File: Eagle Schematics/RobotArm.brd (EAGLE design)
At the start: 54.5 x 52.6 mm, 86 parts, among them J1 5A/28V, SW1 5A/28V

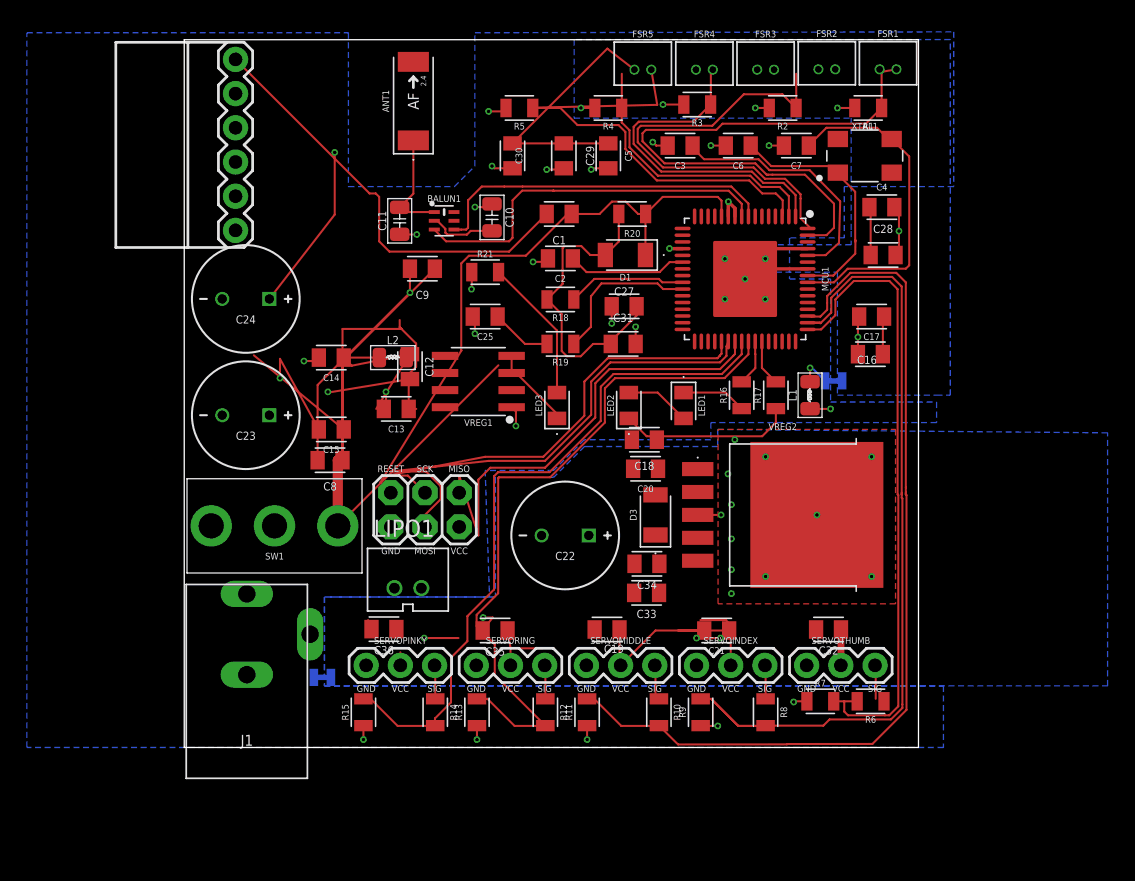
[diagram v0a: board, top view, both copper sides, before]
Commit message: reorganized
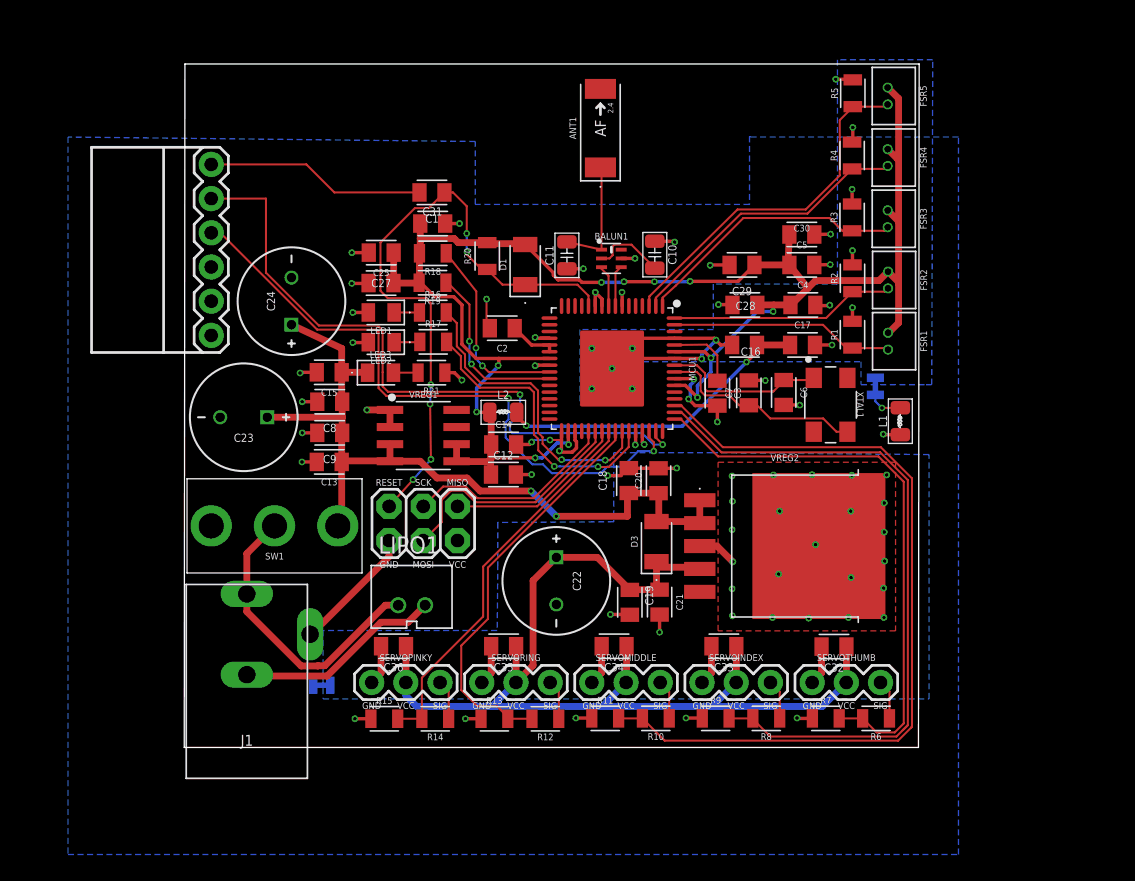
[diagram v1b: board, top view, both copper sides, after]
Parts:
- moved R17 25.8 mm to (18.5, 30.1), turned to 0 degrees
- moved R5 24.8 mm to (49.7, 48.6), turned to 90 degrees
- moved R16 23.7 mm to (18.5, 32.3), turned to 0 degrees
- moved LED1 23.5 mm to (14.6, 32.3), turned to 180 degrees
- moved C30 22.3 mm to (45.9, 38.1), turned to 0 degrees
- moved FSR1 20.2 mm to (52.3, 30.2), turned to 270 degrees
- moved LED2 19.0 mm to (14.6, 30.1), turned to 180 degrees
- moved C7 18.7 mm to (41.9, 26.3), turned to 90 degrees
- moved XTAL1 18.7 mm to (48.0, 25.5), turned to 270 degrees
- moved C6 18.6 mm to (44.5, 26.4), turned to 270 degrees
- moved C3 18.6 mm to (39.6, 26.3), turned to 270 degrees
- moved R4 18.5 mm to (49.6, 44.0), turned to 90 degrees
- moved FSR5 18.3 mm to (52.2, 48.4), turned to 270 degrees
- moved C27 18.1 mm to (14.6, 34.5)
- moved R1 16.9 mm to (49.6, 30.7), turned to 90 degrees
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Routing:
- net VCC: track 63.7 -> 127.2 mm, vias 0 -> 12
- net 5V: track 25.9 -> 80.4 mm
- net TX0: track 0.00 -> 50.6 mm, vias 0 -> 2
- net RX0: track 0.00 -> 47.0 mm, vias 0 -> 2
- net VBAT: track 89.7 -> 60.7 mm, vias 1 -> 2
- net PRESS-THUMB: track 43.0 -> 16.6 mm
- net N$12: track 27.8 -> 3.10 mm
- net N$11: track 25.9 -> 3.08 mm
- net SERVO-PINKY: track 51.1 -> 28.9 mm
- net +: track 0.00 -> 22.0 mm
- net SERVO-RING: track 51.9 -> 30.2 mm
- net MISO: track 35.4 -> 13.8 mm
- net AVCC: track 2.83 -> 23.9 mm, vias 0 -> 2
- net MOSI: track 38.4 -> 18.3 mm
- net PB6: track 3.42 -> 22.9 mm, vias 0 -> 2
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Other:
- board size 54.5 x 52.6 mm -> 54.6 x 50.8 mm
